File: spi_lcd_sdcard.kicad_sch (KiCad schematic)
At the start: 4 parts, among them U8 MAX98357A, U9 ADS1110

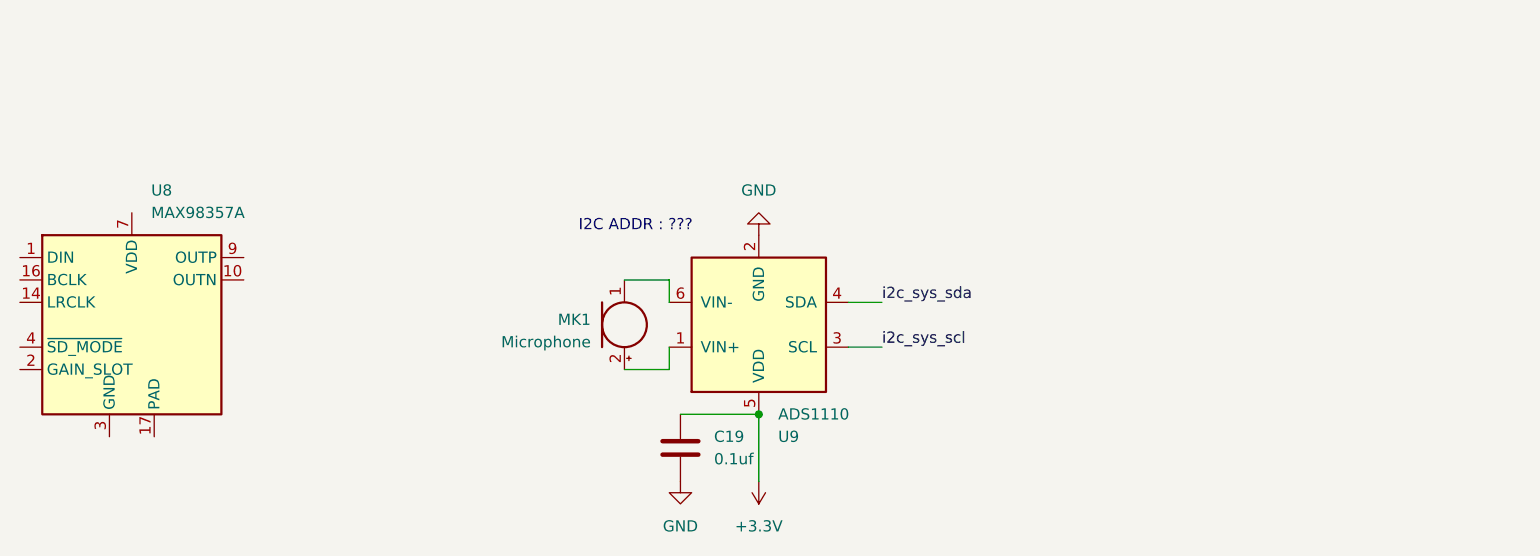
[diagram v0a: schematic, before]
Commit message: initial commit
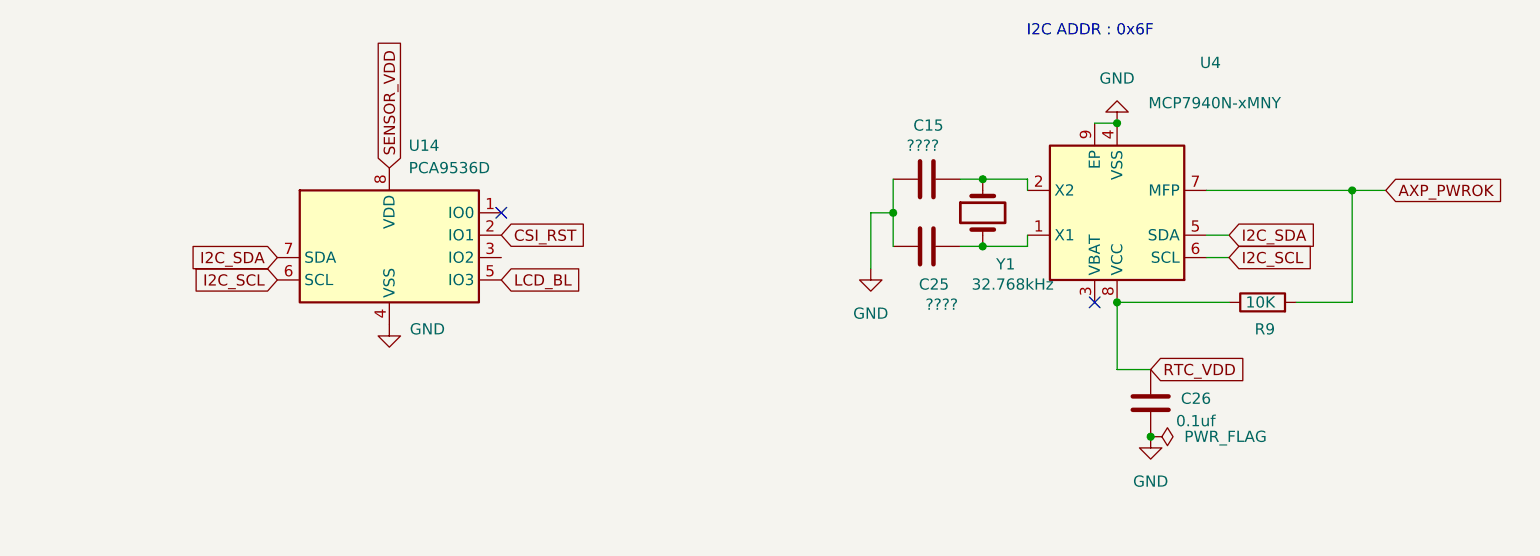
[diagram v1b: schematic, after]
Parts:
- removed C19: 0.1uf, symbol Device:C
- removed MK1: Microphone, symbol Device:Microphone
- removed U8: MAX98357A, Package_DFN_QFN:TQFN-16-1EP_3x3mm_P0.5mm_EP1.23x1.23mm, symbol Audio:MAX98357A
- removed U9: ADS1110, Package_TO_SOT_SMD:SOT-23-6, symbol Analog_ADC:ADS1110
- added C15, C25: ????, Capacitor_SMD:C_0603_1608Metric_Pad1.08x0.95mm_HandSolder, symbol Device:C
- added C26: 0.1uf, Capacitor_SMD:C_0603_1608Metric_Pad1.08x0.95mm_HandSolder, symbol Device:C
- added R9: 10K, Resistor_SMD:R_0603_1608Metric_Pad0.98x0.95mm_HandSolder, symbol Device:R
- added U14: PCA9536D, Package_SO:SOIC-8_3.9x4.9mm_P1.27mm, symbol Interface_Expansion:PCA9536D
- added U4: MCP7940N-xMNY, Package_DFN_QFN:DFN-8-1EP_3x2mm_P0.5mm_EP1.36x1.46mm, symbol Timer_RTC:MCP7940N-xMNY
- added Y1: 32.768kHz, Crystal:Crystal_SMD_3215-2Pin_3.2x1.5mm, symbol Device:Crystal
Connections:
- net GND: now also C15.2, C25.1, C26.2, U14.4 (VSS), U4.4 (VSS), U4.9 (EP)
- new net: C25.2, U4.1 (X1), Y1.2
- new net: C15.1, U4.2 (X2), Y1.1
- new net AXP_PWROK: R9.2, U4.7 (MFP)
- new net CSI_RST: U14.2 (IO1)
- new net I2C_SCL: U14.6 (SCL), U4.6 (SCL)
- new net I2C_SDA: U14.7 (SDA), U4.5 (SDA)
- new net LCD_BL: U14.5 (IO3)
- new net RTC_VDD: C26.1, R9.1, U4.8 (VCC)
- new net SENSOR_VDD: U14.8 (VDD)
- no-connect marks 0 -> 2
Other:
- note added: "I2C ADDR : 0x6F"
- note removed: "I2C ADDR : ???"
- company: (none) -> Buildybee
- title: (none) -> BEEPRO
